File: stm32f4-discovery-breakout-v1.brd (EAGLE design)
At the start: 98.5 x 69.5 mm, 5 parts

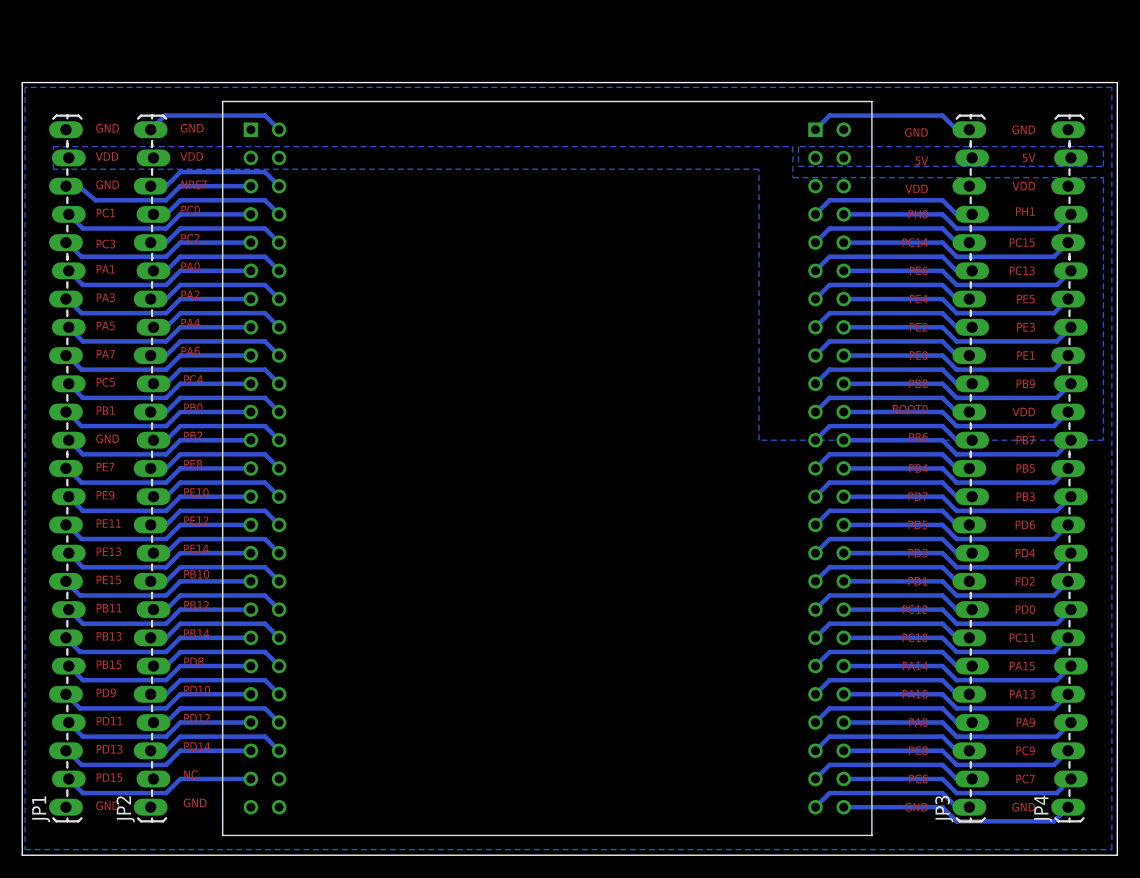
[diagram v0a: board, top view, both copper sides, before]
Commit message: Is this the final?
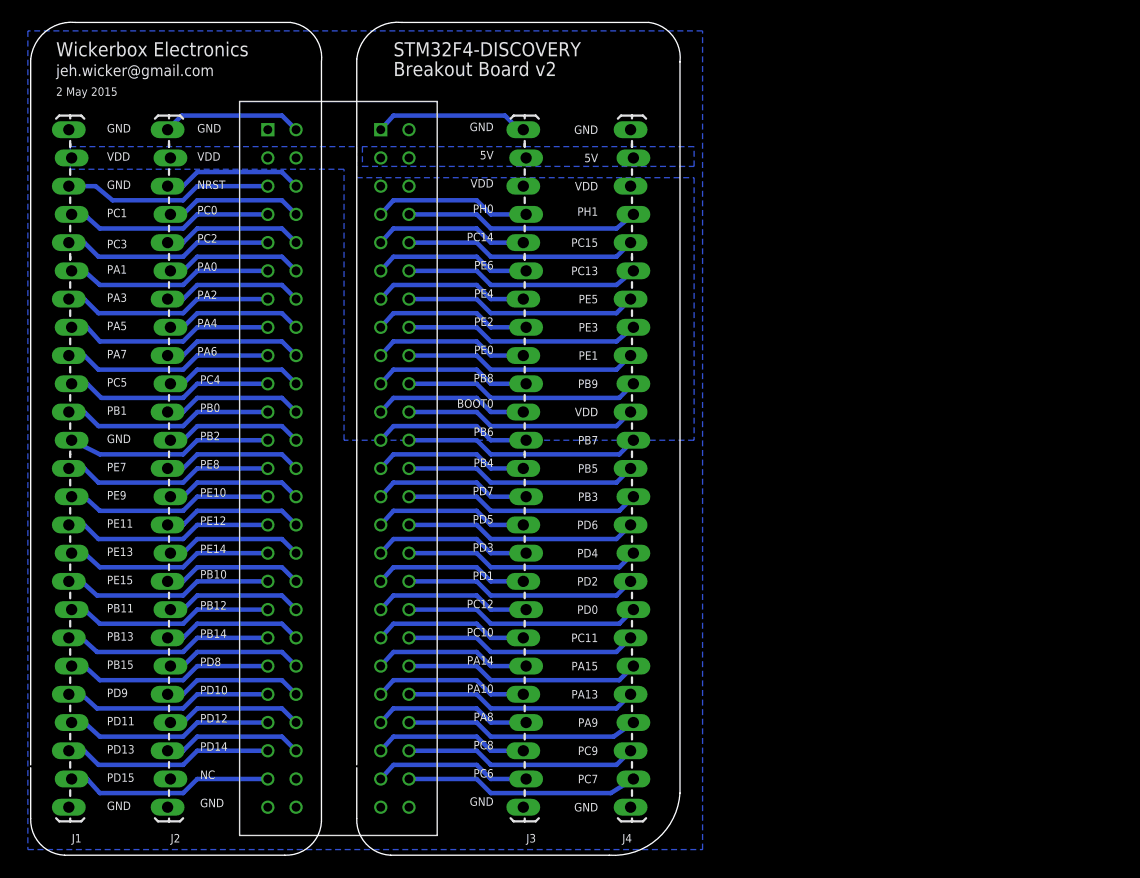
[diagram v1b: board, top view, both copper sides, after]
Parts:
- removed JP1, JP2, JP3, JP4: M25LOCK_LONGPADS, SparkFun-Connectors:1X25_LOCK_LONGPADS
- added J1, J2, J3, J4: (no value), SparkFun-Connectors:1X25_LOCK_LONGPADS
- moved U$1 1.52 mm to (50.0, 34.8)
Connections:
- net 5V: now also J3.24, J4.24; no longer JP3.24, JP4.24
- net BOOT0: now also J3.15; no longer JP3.15
- net GND: now also J1.1, J1.14, J1.23, J1.25, J2.1, J2.25, J3.1, J3.25, J4.1, J4.25; no longer JP1.1, JP1.14, JP1.23, JP1.25, JP2.1, JP2.25, JP3.1, JP3.25, JP4.1, JP4.25
- net NRST: now also J2.23; no longer JP2.23
- net PA0: now also J2.20; no longer JP2.20
- net PA1: now also J1.20; no longer JP1.20
- net PA10: now also J3.5; no longer JP3.5
- net PA13: now also J4.5; no longer JP4.5
- net PA14: now also J3.6; no longer JP3.6
- net PA15: now also J4.6; no longer JP4.6
- net PA2: now also J2.19; no longer JP2.19
- net PA3: now also J1.19; no longer JP1.19
- net PA4: now also J2.18; no longer JP2.18
- net PA5: now also J1.18; no longer JP1.18
- net PA6: now also J2.17; no longer JP2.17
- net PA7: now also J1.17; no longer JP1.17
- net PA8: now also J3.4; no longer JP3.4
- net PA9: now also J4.4; no longer JP4.4
- net PB0: now also J2.15; no longer JP2.15
- net PB1: now also J1.15; no longer JP1.15
- net PB10: now also J2.9; no longer JP2.9
- net PB11: now also J1.8; no longer JP1.8
- net PB12: now also J2.8; no longer JP2.8
- net PB13: now also J1.7; no longer JP1.7
- net PB14: now also J2.7; no longer JP2.7
- net PB15: now also J1.6; no longer JP1.6
- net PB2: now also J2.14; no longer JP2.14
- net PB3: now also J4.12; no longer JP4.12
- net PB4: now also J3.13; no longer JP3.13
- net PB5: now also J4.13; no longer JP4.13
- net PB6: now also J3.14; no longer JP3.14
- net PB7: now also J4.14; no longer JP4.14
- net PB8: now also J3.16; no longer JP3.16
- net PB9: now also J4.16; no longer JP4.16
- net PC0: now also J2.22; no longer JP2.22
- net PC1: now also J1.22; no longer JP1.22
- net PC10: now also J3.7; no longer JP3.7
- net PC11: now also J4.7; no longer JP4.7
- net PC12: now also J3.8; no longer JP3.8
- net PC13: now also J4.20; no longer JP4.20
- net PC14: now also J3.21; no longer JP3.21
- net PC15: now also J4.21; no longer JP4.21
- net PC2: now also J2.21; no longer JP2.21
- net PC3: now also J1.21; no longer JP1.21
- net PC4: now also J2.16; no longer JP2.16
- net PC5: now also J1.16; no longer JP1.16
- net PC6: now also J3.2; no longer JP3.2
- net PC7: now also J4.2; no longer JP4.2
- net PC8: now also J3.3; no longer JP3.3
- net PC9: now also J4.3; no longer JP4.3
- net PD0: now also J4.8; no longer JP4.8
- net PD1: now also J3.9; no longer JP3.9
- net PD10: now also J2.5; no longer JP2.5
- net PD11: now also J1.4; no longer JP1.4
- net PD12: now also J2.4; no longer JP2.4
- net PD13: now also J1.3; no longer JP1.3
- net PD14: now also J2.3; no longer JP2.3
- net PD15: now also J1.2; no longer JP1.2
- net PD2: now also J4.9; no longer JP4.9
- net PD3: now also J3.10; no longer JP3.10
- net PD4: now also J4.10; no longer JP4.10
- net PD5: now also J3.11; no longer JP3.11
- net PD6: now also J4.11; no longer JP4.11
- net PD7: now also J3.12; no longer JP3.12
- net PD8: now also J2.6; no longer JP2.6
- net PD9: now also J1.5; no longer JP1.5
- net PE0: now also J3.17; no longer JP3.17
- net PE1: now also J4.17; no longer JP4.17
- net PE10: now also J2.12; no longer JP2.12
- net PE11: now also J1.11; no longer JP1.11
- net PE12: now also J2.11; no longer JP2.11
- net PE13: now also J1.10; no longer JP1.10
- net PE14: now also J2.10; no longer JP2.10
- net PE15: now also J1.9; no longer JP1.9
- net PE2: now also J3.18; no longer JP3.18
- net PE3: now also J4.18; no longer JP4.18
- net PE4: now also J3.19; no longer JP3.19
- net PE5: now also J4.19; no longer JP4.19
- net PE6: now also J3.20; no longer JP3.20
- net PE7: now also J1.13; no longer JP1.13
- net PE8: now also J2.13; no longer JP2.13
- net PE9: now also J1.12; no longer JP1.12
- net PH0: now also J3.22; no longer JP3.22
- net PH1: now also J4.22; no longer JP4.22
- net VDD: now also J1.24, J2.24, J3.23, J4.15, J4.23; no longer JP1.24, JP2.24, JP3.23, JP4.15, JP4.23
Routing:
- net GND: track 98.7 -> 63.9 mm
- net PD15: track 17.4 -> 18.7 mm
- net PA5: track 17.4 -> 18.7 mm
- net PA7: track 17.7 -> 19.0 mm
- net PA3: track 17.7 -> 19.0 mm
- net PE7: track 17.7 -> 19.0 mm
- net PE11: track 17.7 -> 19.0 mm
- net PD13: track 17.7 -> 19.0 mm
- net PC5: track 17.4 -> 18.7 mm
- net PC3: track 17.7 -> 19.0 mm
- net PB1: track 17.7 -> 19.0 mm
- net PA1: track 17.4 -> 18.7 mm
- net PC1: track 17.4 -> 18.7 mm
- net PE9: track 17.4 -> 18.7 mm
- net PE15: track 17.7 -> 18.9 mm
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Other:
- board size 98.5 x 69.5 mm -> 58.4 x 75 mm
- board text added: "2 May 2015"
- board text added: "Breakout Board v2"
- board text added: "STM32F4-DISCOVERY"
- board text added: "Wickerbox Electronics"
- board text added: "jeh.wicker@gmail.com"

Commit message: Fixed up version numbers.
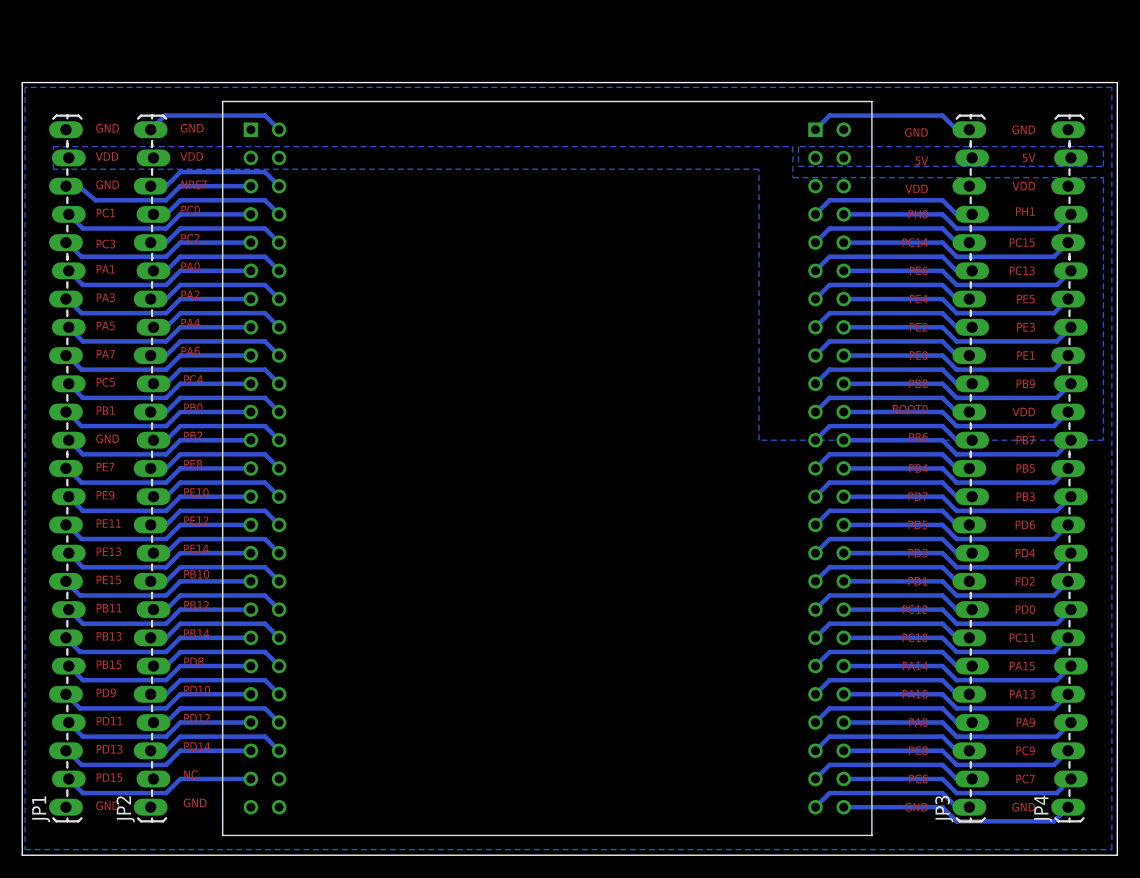
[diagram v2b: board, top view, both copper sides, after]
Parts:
- removed J1, J2, J3, J4: (no value), SparkFun-Connectors:1X25_LOCK_LONGPADS
- added JP1, JP2, JP3, JP4: M25LOCK_LONGPADS, SparkFun-Connectors:1X25_LOCK_LONGPADS
- moved U$1 1.52 mm to (48.5, 34.8)
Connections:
- net 5V: now also JP3.24, JP4.24; no longer J3.24, J4.24
- net BOOT0: now also JP3.15; no longer J3.15
- net GND: now also JP1.1, JP1.14, JP1.23, JP1.25, JP2.1, JP2.25, JP3.1, JP3.25, JP4.1, JP4.25; no longer J1.1, J1.14, J1.23, J1.25, J2.1, J2.25, J3.1, J3.25, J4.1, J4.25
- net NRST: now also JP2.23; no longer J2.23
- net PA0: now also JP2.20; no longer J2.20
- net PA1: now also JP1.20; no longer J1.20
- net PA10: now also JP3.5; no longer J3.5
- net PA13: now also JP4.5; no longer J4.5
- net PA14: now also JP3.6; no longer J3.6
- net PA15: now also JP4.6; no longer J4.6
- net PA2: now also JP2.19; no longer J2.19
- net PA3: now also JP1.19; no longer J1.19
- net PA4: now also JP2.18; no longer J2.18
- net PA5: now also JP1.18; no longer J1.18
- net PA6: now also JP2.17; no longer J2.17
- net PA7: now also JP1.17; no longer J1.17
- net PA8: now also JP3.4; no longer J3.4
- net PA9: now also JP4.4; no longer J4.4
- net PB0: now also JP2.15; no longer J2.15
- net PB1: now also JP1.15; no longer J1.15
- net PB10: now also JP2.9; no longer J2.9
- net PB11: now also JP1.8; no longer J1.8
- net PB12: now also JP2.8; no longer J2.8
- net PB13: now also JP1.7; no longer J1.7
- net PB14: now also JP2.7; no longer J2.7
- net PB15: now also JP1.6; no longer J1.6
- net PB2: now also JP2.14; no longer J2.14
- net PB3: now also JP4.12; no longer J4.12
- net PB4: now also JP3.13; no longer J3.13
- net PB5: now also JP4.13; no longer J4.13
- net PB6: now also JP3.14; no longer J3.14
- net PB7: now also JP4.14; no longer J4.14
- net PB8: now also JP3.16; no longer J3.16
- net PB9: now also JP4.16; no longer J4.16
- net PC0: now also JP2.22; no longer J2.22
- net PC1: now also JP1.22; no longer J1.22
- net PC10: now also JP3.7; no longer J3.7
- net PC11: now also JP4.7; no longer J4.7
- net PC12: now also JP3.8; no longer J3.8
- net PC13: now also JP4.20; no longer J4.20
- net PC14: now also JP3.21; no longer J3.21
- net PC15: now also JP4.21; no longer J4.21
- net PC2: now also JP2.21; no longer J2.21
- net PC3: now also JP1.21; no longer J1.21
- net PC4: now also JP2.16; no longer J2.16
- net PC5: now also JP1.16; no longer J1.16
- net PC6: now also JP3.2; no longer J3.2
- net PC7: now also JP4.2; no longer J4.2
- net PC8: now also JP3.3; no longer J3.3
- net PC9: now also JP4.3; no longer J4.3
- net PD0: now also JP4.8; no longer J4.8
- net PD1: now also JP3.9; no longer J3.9
- net PD10: now also JP2.5; no longer J2.5
- net PD11: now also JP1.4; no longer J1.4
- net PD12: now also JP2.4; no longer J2.4
- net PD13: now also JP1.3; no longer J1.3
- net PD14: now also JP2.3; no longer J2.3
- net PD15: now also JP1.2; no longer J1.2
- net PD2: now also JP4.9; no longer J4.9
- net PD3: now also JP3.10; no longer J3.10
- net PD4: now also JP4.10; no longer J4.10
- net PD5: now also JP3.11; no longer J3.11
- net PD6: now also JP4.11; no longer J4.11
- net PD7: now also JP3.12; no longer J3.12
- net PD8: now also JP2.6; no longer J2.6
- net PD9: now also JP1.5; no longer J1.5
- net PE0: now also JP3.17; no longer J3.17
- net PE1: now also JP4.17; no longer J4.17
- net PE10: now also JP2.12; no longer J2.12
- net PE11: now also JP1.11; no longer J1.11
- net PE12: now also JP2.11; no longer J2.11
- net PE13: now also JP1.10; no longer J1.10
- net PE14: now also JP2.10; no longer J2.10
- net PE15: now also JP1.9; no longer J1.9
- net PE2: now also JP3.18; no longer J3.18
- net PE3: now also JP4.18; no longer J4.18
- net PE4: now also JP3.19; no longer J3.19
- net PE5: now also JP4.19; no longer J4.19
- net PE6: now also JP3.20; no longer J3.20
- net PE7: now also JP1.13; no longer J1.13
- net PE8: now also JP2.13; no longer J2.13
- net PE9: now also JP1.12; no longer J1.12
- net PH0: now also JP3.22; no longer J3.22
- net PH1: now also JP4.22; no longer J4.22
- net VDD: now also JP1.24, JP2.24, JP3.23, JP4.15, JP4.23; no longer J1.24, J2.24, J3.23, J4.15, J4.23
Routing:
- net GND: track 63.9 -> 98.7 mm
- net PD15: track 18.7 -> 17.4 mm
- net PA5: track 18.7 -> 17.4 mm
- net PA7: track 19.0 -> 17.7 mm
- net PA3: track 19.0 -> 17.7 mm
- net PE7: track 19.0 -> 17.7 mm
- net PE11: track 19.0 -> 17.7 mm
- net PD13: track 19.0 -> 17.7 mm
- net PC5: track 18.7 -> 17.4 mm
- net PC3: track 19.0 -> 17.7 mm
- net PB1: track 19.0 -> 17.7 mm
- net PA1: track 18.7 -> 17.4 mm
- net PC1: track 18.7 -> 17.4 mm
- net PE9: track 18.7 -> 17.4 mm
- net PE15: track 18.9 -> 17.7 mm
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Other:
- board size 58.4 x 75 mm -> 98.5 x 69.5 mm
- board text removed: "2 May 2015"
- board text removed: "Breakout Board v2"
- board text removed: "STM32F4-DISCOVERY"
- board text removed: "Wickerbox Electronics"
- board text removed: "jeh.wicker@gmail.com"
